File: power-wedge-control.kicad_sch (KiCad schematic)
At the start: 58 parts, among them J1 Conn_01x02, J2 Conn_01x03, J3 Conn_01x02, J4 Conn_01x03, J5 Conn_01x03, J6 Conn_01x06_Female, J7 Conn_01x04_Female, J8 Conn_01x03, J9 MicroSD_Hirose_DM3D-SF, Q1 MMBT3904L, Q2 DMP3099L, Q3 MMBT3904L, Q4 DMP3099L, Q5 MMBT3904L, Q6 MMBT3904L, U1 LM1117-5.0, U3 TLV70233DBV, U5 NC7WZ17P6X, U6 NC7WZ17P6X

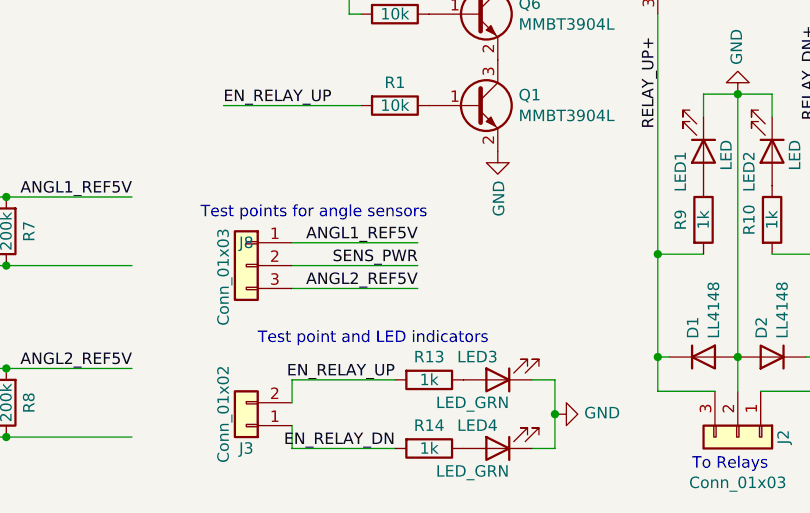
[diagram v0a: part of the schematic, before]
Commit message: Add GND to angle sensor test points.
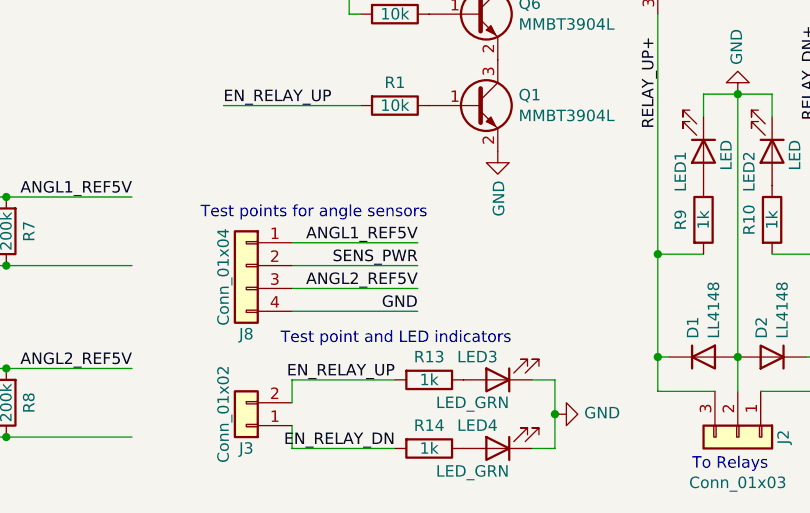
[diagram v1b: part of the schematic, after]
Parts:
- J8: value Conn_01x03 -> Conn_01x04; footprint Connector_PinHeader_2.54mm:PinHeader_1x03_P2.54mm_Horizontal -> Connector_PinHeader_2.54mm:PinHeader_1x04_P2.54mm_Horizontal; symbol Connector_Generic:Conn_01x03 -> Connector_Generic:Conn_01x04
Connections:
- net GND: now also J8.4 (Pin_4)
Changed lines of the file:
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@@
+    (stroke (width 0) (type default) (color 0 0 0 0))
+  )
+  (wire (pts (xy 114.3 177.8) (xy 128.27 177.8))
     (stroke (width 0) (type default) (color 0 0 0 0))
   )
@@
     (effects (font (size 1.524 1.524)) (justify left bottom))
   )
-  (text "Test point and LED indicators" (at 110.49 181.61 0)
+  (text "Test point and LED indicators" (at 113.03 181.61 0)
     (effects (font (size 1.27 1.27)) (justify left bottom))
   )
@@
   (label "BTN_PWR" (at 24.13 83.82 0)
     (effects (font (size 1.27 1.27)) (justify left bottom))
+  )
+  (label "GND" (at 128.27 177.8 180)
+    (effects (font (size 1.27 1.27)) (justify right bottom))
   )
   (label "EN_OUTPUT" (at 106.68 113.03 0)
@@
     (pin "2")
   )
-  (symbol (lib_id "Connector_Generic:Conn_01x03") (at 109.22 172.72 0) (mirror y) (unit 1)
-    (in_bom yes) (on_board yes)
-    (property "Reference" "J8" (id 0) (at 109.22 170.18 0))
-    (property "Value" "Conn_01x03" (id 1) (at 106.68 173.99 90))
-    (property "Footprint" "Connector_PinHeader_2.54mm:PinHeader_1x03_P2.54mm_Horizontal" (id 2) (at 109.22 172.72 0)
+  (symbol (lib_id "Connector_Generic:Conn_01x04") (at 109.22 172.72 0) (mirror y) (unit 1)
+    (in_bom yes) (on_board yes)
+    (property "Reference" "J8" (id 0) (at 109.22 180.34 0))
+    (property "Value" "Conn_01x04" (id 1) (at 106.68 173.99 90))
+    (property "Footprint" "Connector_PinHeader_2.54mm:PinHeader_1x04_P2.54mm_Horizontal" (id 2) (at 109.22 172.72 0)
       (effects (font (size 1.27 1.27)) hide)
     )
@@
     (pin "2")
     (pin "3")
+    (pin "4")
   )
   (symbol (lib_id "Connector:Conn_01x04_Female") (at 21.59 91.44 0) (mirror y) (unit 1)
@@
     )
     (path "/4525ae04-c30a-4c84-af19-511fb2ef01b1"
-      (reference "J8") (unit 1) (value "Conn_01x03") (footprint "Connector_PinHeader_2.54mm:PinHeader_1x03_P2.54mm_Horizontal")
+      (reference "J8") (unit 1) (value "Conn_01x04") (footprint "Connector_PinHeader_2.54mm:PinHeader_1x04_P2.54mm_Horizontal")
     )
     (path "/aa36bbf1-be88-483c-a548-fa695999538f"

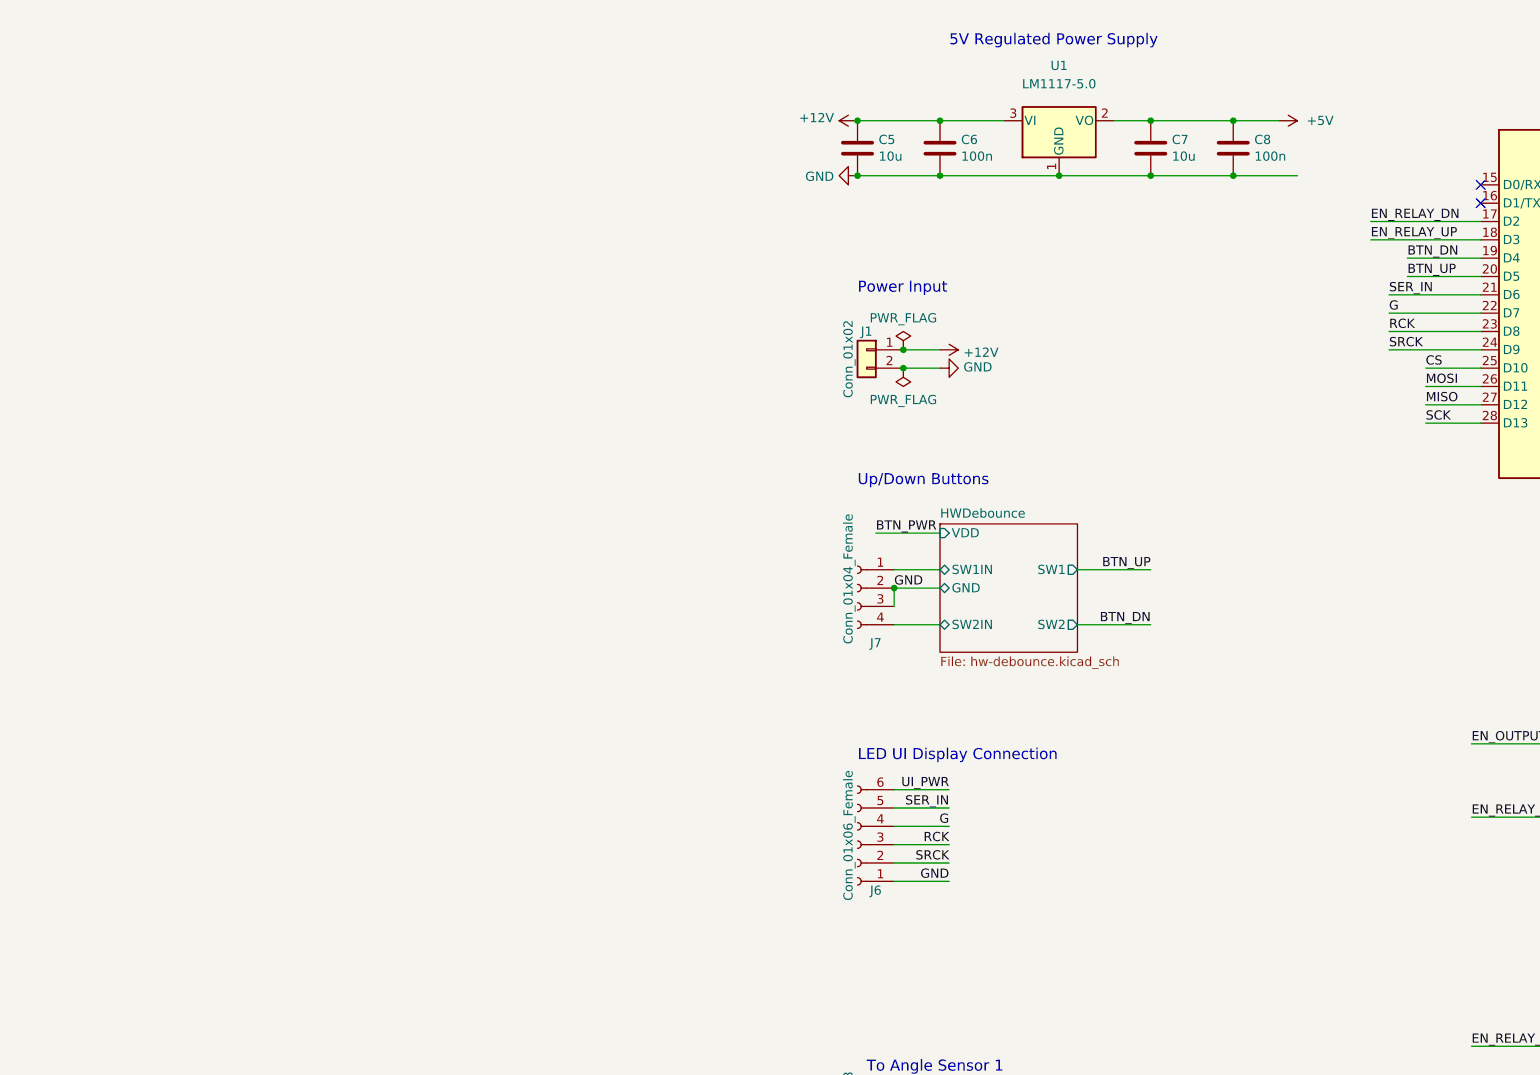
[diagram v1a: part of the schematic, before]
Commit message: WIP. Add support for active-high (15V max) switch input to schematic.
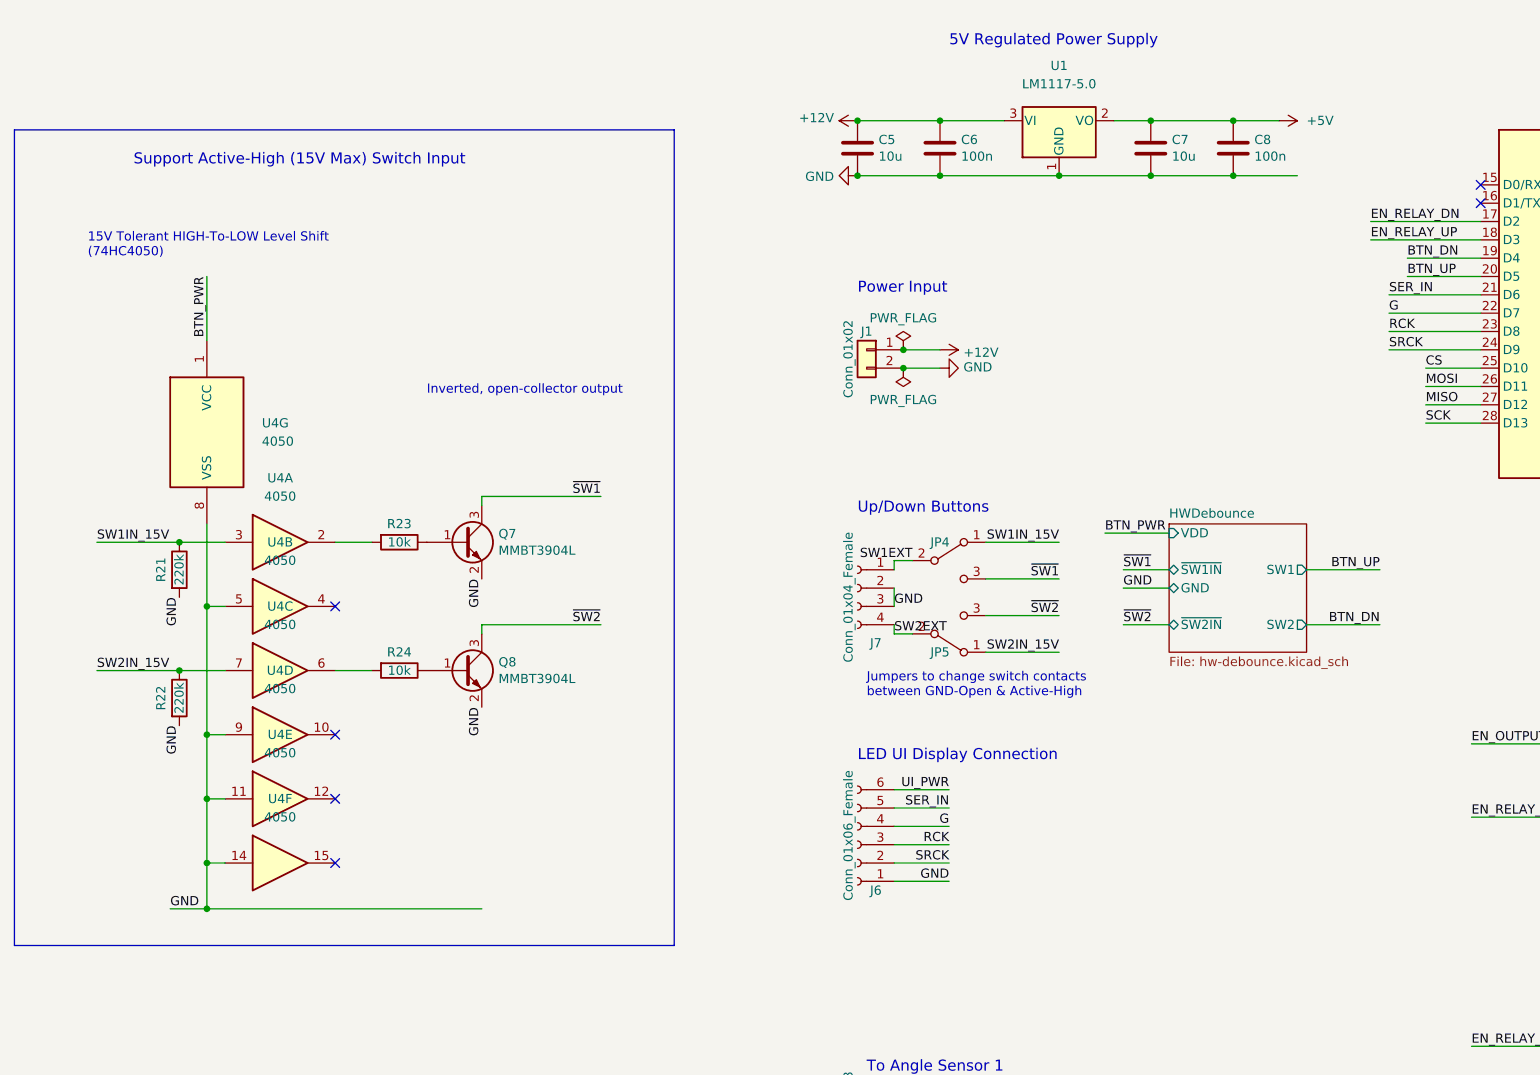
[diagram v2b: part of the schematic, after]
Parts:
- added JP4, JP5: SW_SPDT, Jumper:SolderJumper-3_P2.0mm_Open_TrianglePad1.0x1.5mm, symbol Switch:SW_SPDT
- added Q7, Q8: MMBT3904L, Package_TO_SOT_SMD:SOT-23, symbol Device:Q_NPN_BEC
- added R21, R22: 220k, Resistor_SMD:R_0603_1608Metric, symbol Device:R
- added R23, R24: 10k, Resistor_SMD:R_0603_1608Metric, symbol Device:R
- added U4: 4050, Package_SO:SOIC-16W_5.3x10.2mm_P1.27mm, symbol 4xxx:4050
- U3: footprint SOT-23-5 -> Package_TO_SOT_SMD:SOT-23-5
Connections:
- net BTN_PWR: now also U4.1 (VCC)
- net GND: now also Q7.2 (E), Q8.2 (E), R21.2, R22.2, U4.11, U4.14, U4.5, U4.8 (VSS), U4.9
- net HWDebounce/SW1IN renamed SW1EXT
- net SW1EXT: now also JP4.2 (B)
- net HWDebounce/SW2IN renamed SW2EXT
- net SW2EXT: now also JP5.2 (B)
- new net: Q8.1 (B), R24.1
- new net: R24.2, U4.6
- new net: R23.2, U4.2
- new net: Q7.1 (B), R23.1
- new net SW1IN_15V: JP4.1 (A), R21.1, U4.3
- new net SW2IN_15V: JP5.1 (A), R22.1, U4.7
- new net ~{SW1}: JP4.3 (C), Q7.3 (C)
- new net ~{SW2}: JP5.3 (C), Q8.3 (C)
- no-connect marks 43 -> 47
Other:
- sheet HWDebounce ports: added ~{SW1IN}, ~{SW2IN}; removed SW1IN, SW2IN
- note added: "15V Tolerant HIGH-To-LOW Level Shift (74HC4050)"
- note added: "Inverted, open-collector output"
- note added: "Jumpers to change switch contacts between GND-Open & Active-High"
- note added: "Support Active-High (15V Max) Switch Input"
